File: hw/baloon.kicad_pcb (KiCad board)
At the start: 2 copper layers, 23.6 x 43.6 mm, 66 parts, among them J1 SOLAR, J2 DEBUG, J3 SWO, J4 ANT, J5 ANT, Q1 BC847, Q2 BC857, Q3 DMP2035, U1 STM32F030C8Tx, U2 Si7020-A20, U3 MS5607-02BA, U4 RFM95W-868S2, U5 MAX-8C/SIM28ML, U6 MCP1640, U7 MCP101-270D, U8 MCP1640

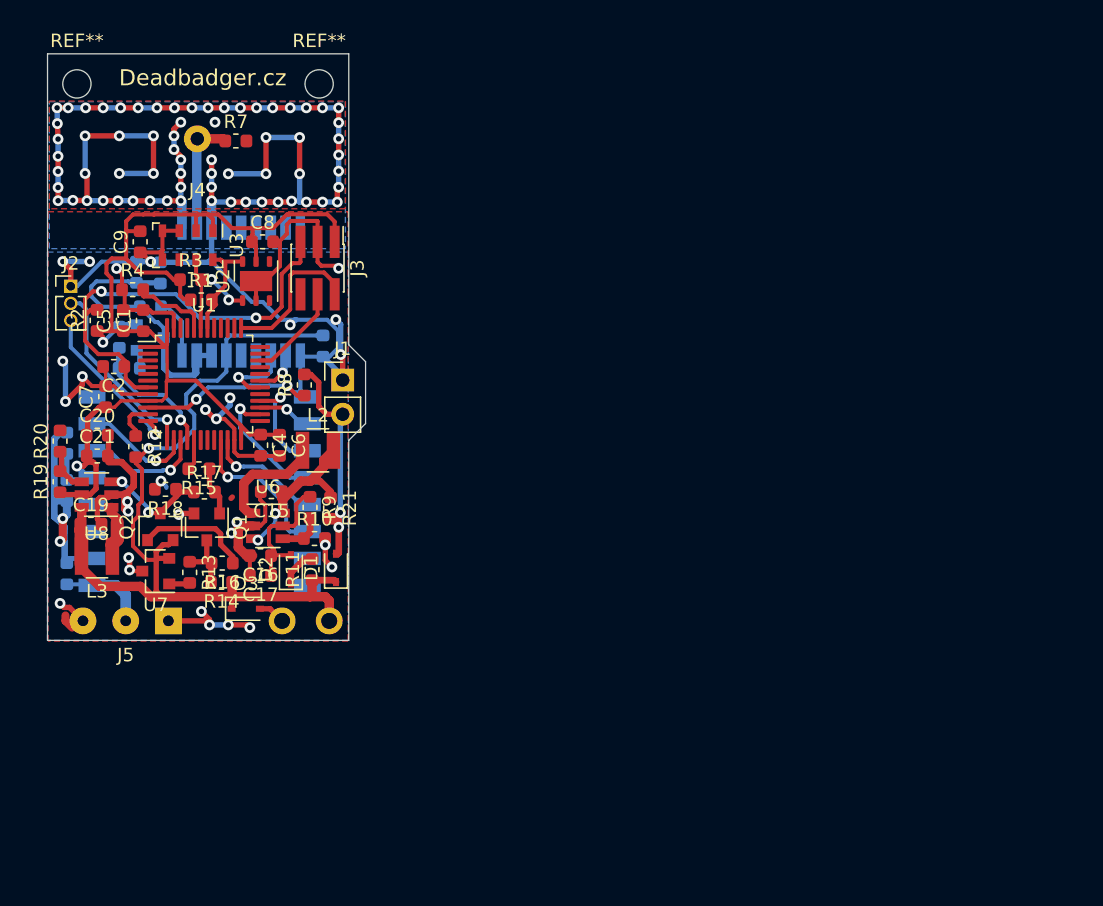
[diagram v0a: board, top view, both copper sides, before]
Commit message: Final board
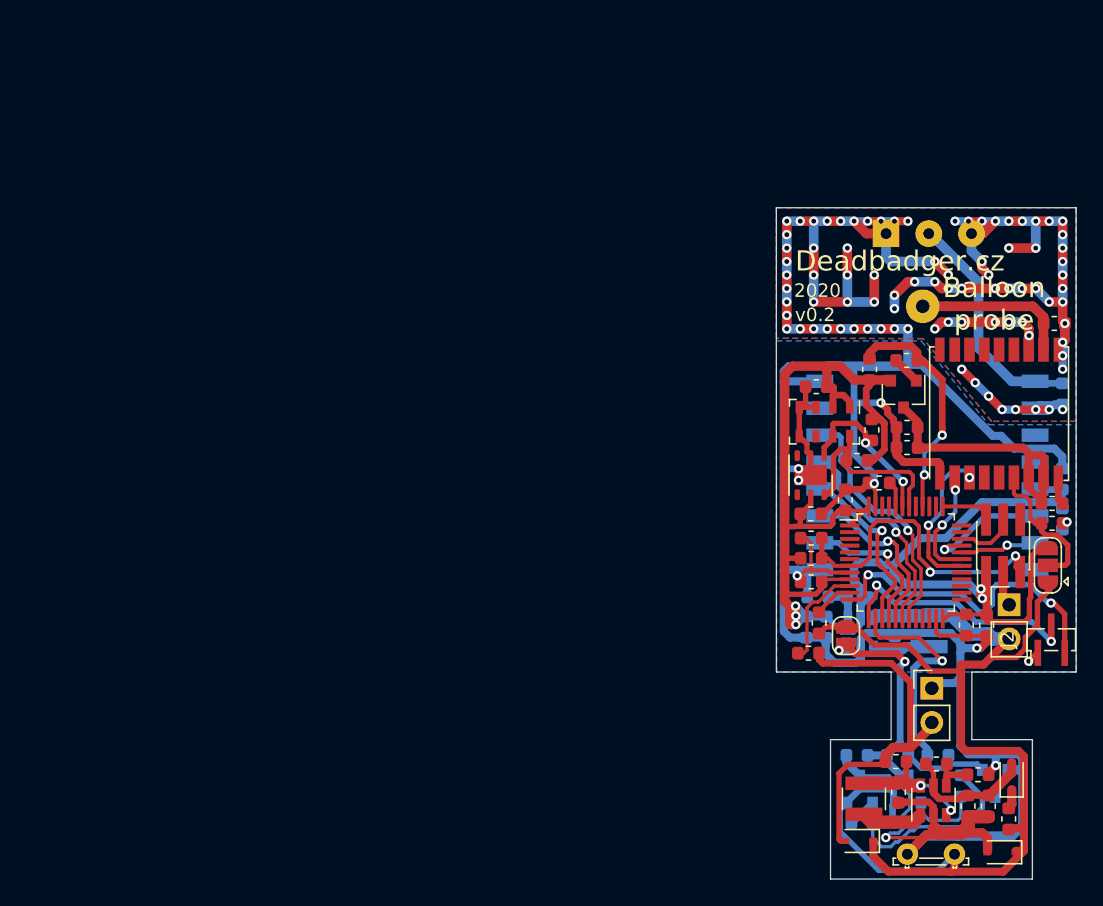
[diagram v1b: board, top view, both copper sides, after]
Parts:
- removed C5: 1u, Capacitor_SMD:C_0603_1608Metric
- removed REF** (x2): MountingHole_2.1mm, MountingHole:MountingHole_2.1mm
- added J6: BAT, Connector_PinHeader_2.54mm:PinHeader_1x02_P2.54mm_Vertical, F.Cu at (155.0, 108.5)
- added JP1: backup, Jumper:SolderJumper-3_P1.3mm_Open_RoundedPad1.0x1.5mm, F.Cu at (157.9, 105.6)
- added JP2: EN, Jumper:SolderJumper-2_P1.3mm_Open_RoundedPad1.0x1.5mm, F.Cu at (142.9, 110.8)
- C12, C13, C14, Q3, R22, R23, R5, U5: moved to F.Cu
- C18: footprint Connector_Phoenix_MC:PhoenixContact_MC_1,5_2-G-3.5_1x02_P3.50mm_Horizontal -> OptoDevice:R_LDR_5.2x5.2mm_P3.5mm_Horizontal; moved to F.Cu
- C19, C20, C21, L3, Q1, Q2, R13, R14, R15, R16, R17, R18, R19, R20, U7, U8: moved to B.Cu
- J2: footprint Connector_PinHeader_1.27mm:PinHeader_1x03_P1.27mm_Vertical -> Connector_PinSocket_1.00mm:PinSocket_1x03_P1.00mm_Vertical_SMD_Pin1Left
- moved J2 77.4 mm to (158.2, 111.1), turned to 90 degrees
- moved R6 75.2 mm to (159.0, 92.8), turned to 270 degrees
- moved C11 74.0 mm to (159.0, 99.2)
- moved C10 74.0 mm to (159.0, 102.1)
- moved R5 68.6 mm to (158.2, 101.0)
- moved C1 66.6 mm to (153.3, 110.0), turned to 270 degrees
- moved R7 62.3 mm to (158.4, 87.6)
- moved L3 62.1 mm to (149.1, 110.5), turned to 270 degrees
- moved Q1 61.6 mm to (154.0, 121.8)
- moved J5 60.6 mm to (145.9, 80.9), turned to 0 degrees
- moved C19 60.2 mm to (146.5, 110.1), turned to 270 degrees
- moved R19 59.9 mm to (143.8, 108.0), turned to 180 degrees
- moved D3 59.0 mm to (154.4, 126.9), turned to 180 degrees
- moved R15 58.9 mm to (149.7, 119.7)
- moved Q2 58.9 mm to (147.5, 122.2)
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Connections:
- C14 pad 2: +BATT -> Net-(C14-Pad2)
- J3 pad 6: Net-(J3-Pad6) -> (no net)
- U1 pad 14: /RFM_IO1 -> /~POWER_OFF
- U1 pad 15: /RFM_IO0 -> /SCK
- U1 pad 16: /~GPS_POWER -> /MISO
- U1 pad 17: /~POWER_OFF -> /MOSI
- U1 pad 18: Net-(U1-Pad18) -> /RFM_CS
- U1 pad 19: Net-(U1-Pad19) -> /RFM_RESET
- U1 pad 2: Net-(U1-Pad2) -> (no net)
- U1 pad 20: Net-(U1-Pad20) -> (no net)
- U1 pad 21: /RFM_RESET -> (no net)
- U1 pad 22: /RFM_CS -> (no net)
- U1 pad 25: Net-(U1-Pad25) -> (no net)
- U1 pad 26: /SCK -> (no net)
- U1 pad 27: /MISO -> (no net)
- U1 pad 28: /MOSI -> (no net)
- U1 pad 29: Net-(U1-Pad29) -> (no net)
- U1 pad 3: Net-(U1-Pad3) -> (no net)
- U1 pad 32: Net-(U1-Pad32) -> /RFM_IO1
- U1 pad 33: Net-(U1-Pad33) -> /RFM_IO0
- U1 pad 35: Net-(U1-Pad35) -> (no net)
- U1 pad 36: Net-(U1-Pad36) -> (no net)
- U1 pad 38: Net-(U1-Pad38) -> (no net)
- U1 pad 39: Net-(U1-Pad39) -> (no net)
- U1 pad 4: Net-(U1-Pad4) -> (no net)
- U1 pad 40: Net-(U1-Pad40) -> /~GPS_POWER
- U1 pad 41: Net-(U1-Pad41) -> (no net)
- U1 pad 45: Net-(U1-Pad45) -> (no net)
- U1 pad 46: Net-(U1-Pad46) -> (no net)
- U1 pad 5: Net-(U1-Pad5) -> (no net)
- U1 pad 6: Net-(U1-Pad6) -> (no net)
- U2 pad 3: Net-(U2-Pad3) -> (no net)
- U2 pad 4: Net-(U2-Pad4) -> (no net)
- U3 pad 6: Net-(U3-Pad6) -> (no net)
- U4 pad 11: Net-(U4-Pad11) -> (no net)
- U4 pad 12: Net-(U4-Pad12) -> (no net)
- U4 pad 16: Net-(U4-Pad16) -> (no net)
- U4 pad 7: Net-(U4-Pad7) -> (no net)
- U5 pad 13: Net-(U5-Pad13) -> (no net)
- U5 pad 14: Net-(U5-Pad14) -> (no net)
- U5 pad 15: Net-(U5-Pad15) -> (no net)
- U5 pad 16: Net-(U5-Pad16) -> (no net)
- U5 pad 17: Net-(U5-Pad17) -> (no net)
- U5 pad 18: Net-(U5-Pad18) -> (no net)
- U5 pad 4: Net-(U5-Pad4) -> (no net)
- U5 pad 5: Net-(U5-Pad5) -> (no net)
- U5 pad 6: +BATT -> Net-(C14-Pad2)
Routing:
- net GND: track 251.2 -> 312.6 mm, vias 98 -> 96
- net +3V3: track 89.6 -> 122.8 mm, vias 2 -> 5
- net +BATT: track 67.7 -> 90.1 mm, vias 1 -> 0
- net /~POWER_OFF: track 2.31 -> 16.2 mm, vias 0 -> 1
- net /DEBUG_TX: track 12.3 -> 24.0 mm, vias 1 -> 2
- net Net-(J5-Pad2): track 6.80 -> 17.8 mm
- net Net-(C14-Pad2): track 0.00 -> 10.6 mm
- net Net-(Q1-Pad3): track 4.95 -> 15.3 mm
- net Net-(JP2-Pad2): track 8.53 -> 17.8 mm
- net /RESET: track 32.7 -> 23.7 mm
- net /power/Vin: track 17.9 -> 26.7 mm, vias 2 -> 0
- net /SWCLK: track 11.3 -> 3.61 mm
- net /~GPS_POWER: track 10.0 -> 17.5 mm, vias 1 -> 2
- net /RFM_CS: track 8.69 -> 16.1 mm
- net /MISO: track 4.01 -> 11.2 mm
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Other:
- board size 23.6 x 43.6 mm -> 22.3 x 49.9 mm
- board text added: "2020"
- board text added: "Balloon probe"
- board text added: "v0.2"
- board text removed: "Picoballoon v0.1 2020"
